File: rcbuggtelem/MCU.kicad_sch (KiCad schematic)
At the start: 12 parts, among them J3 Micro_SD_Card, J4 USB_B_Micro, U1 ESP32-S3-MINI-1

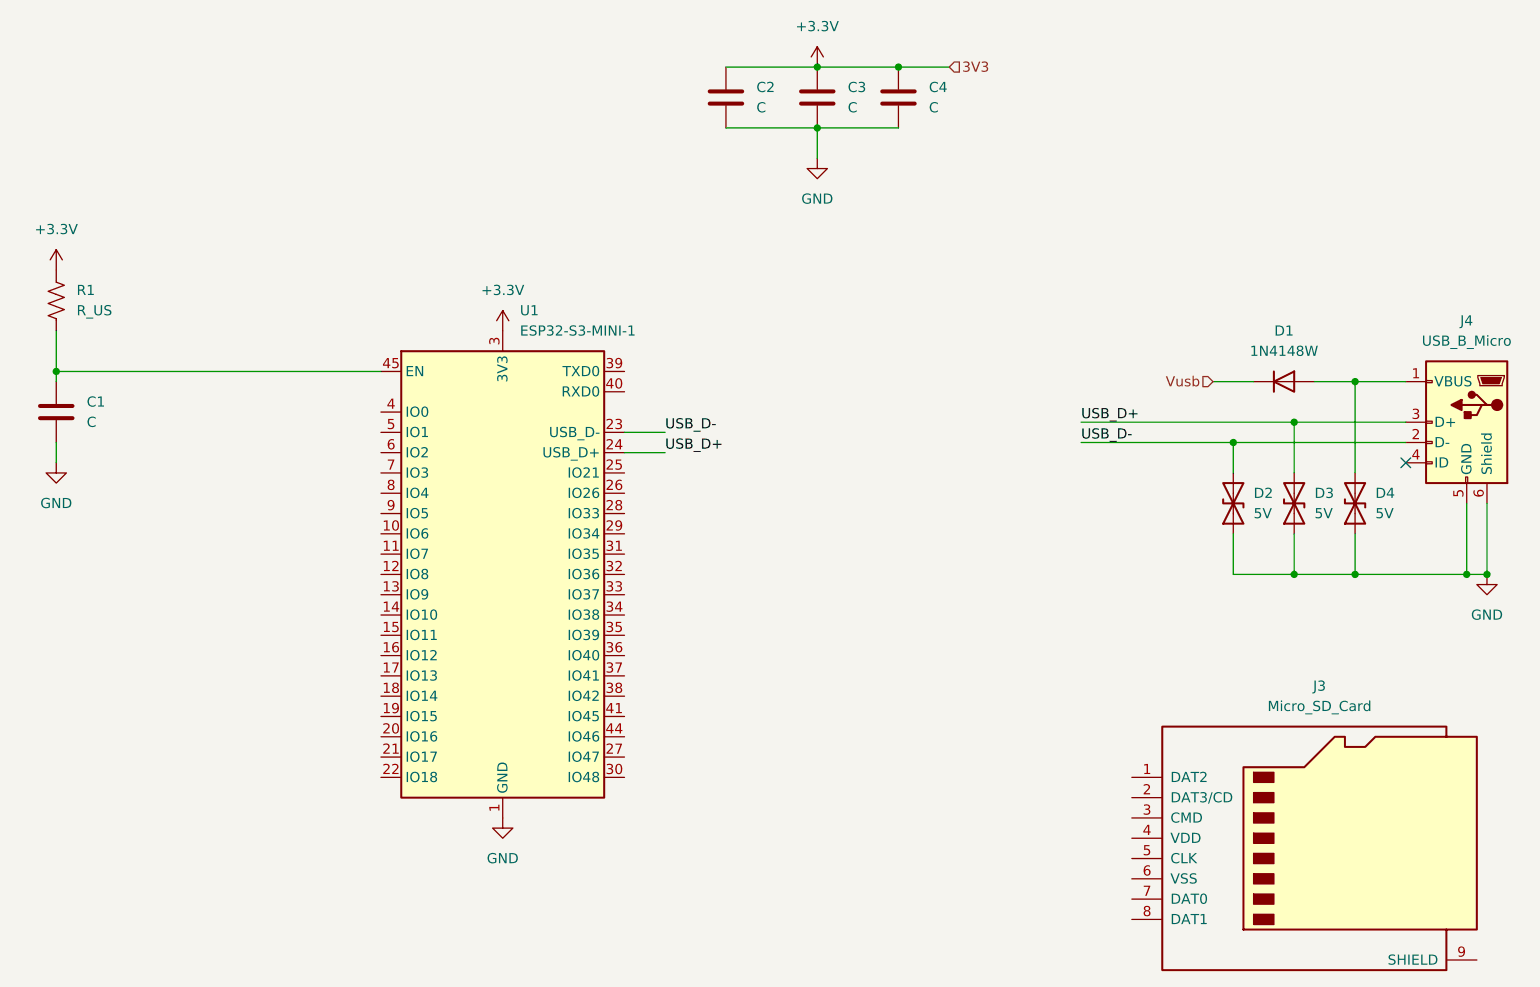
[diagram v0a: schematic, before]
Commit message: Signed-off-by: tom <visentin.tom@gmail.com>
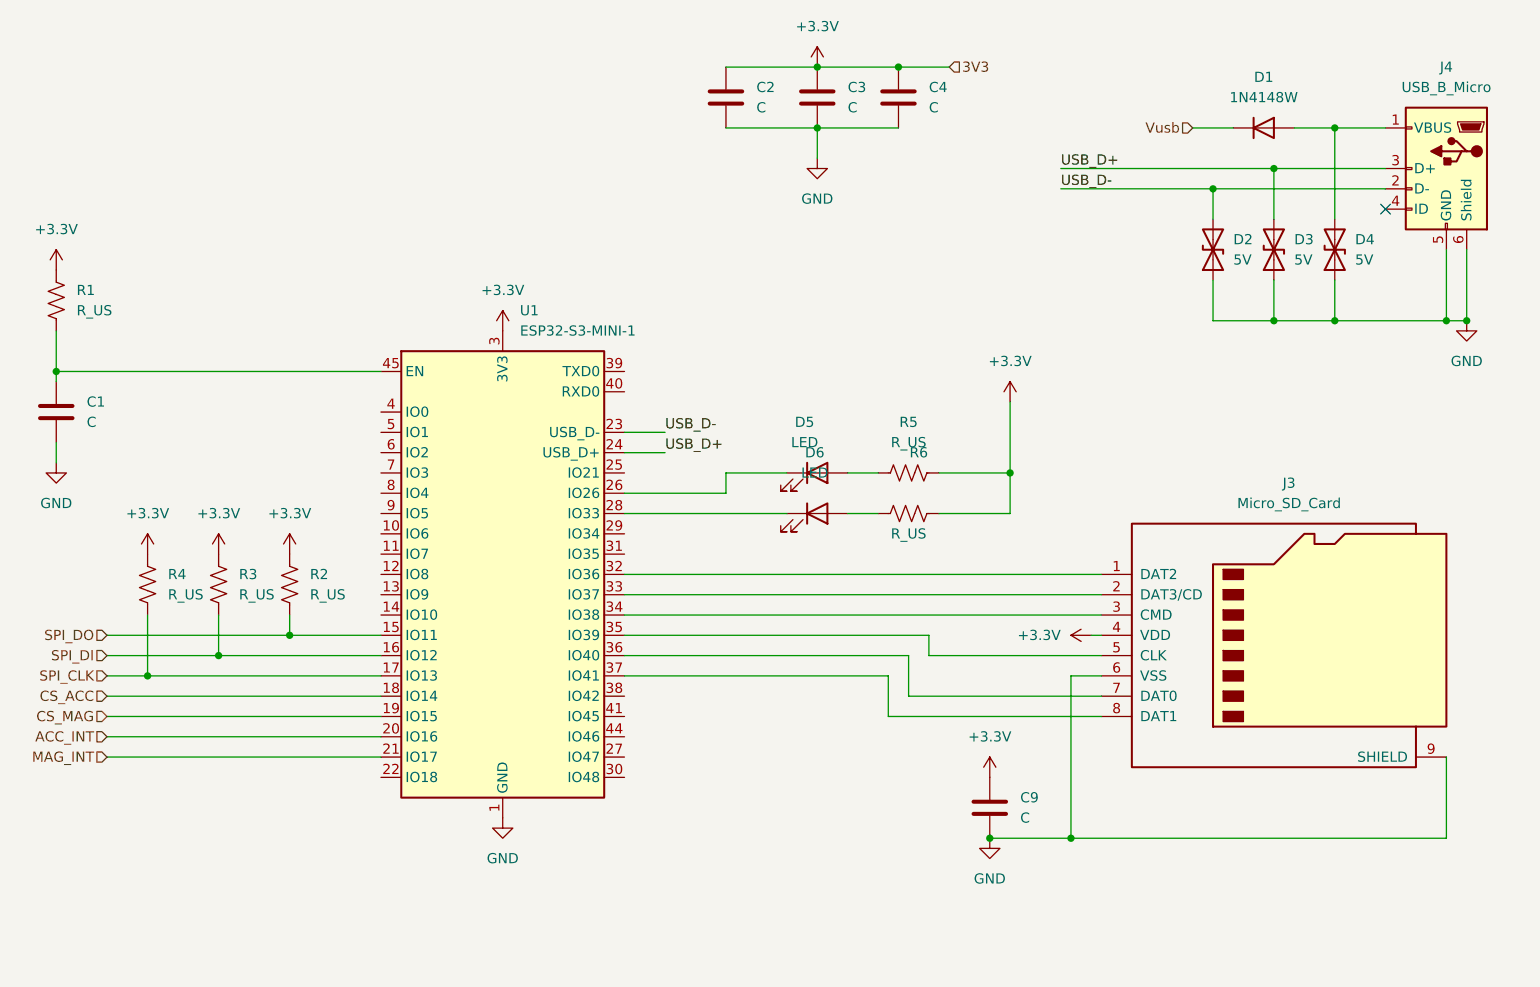
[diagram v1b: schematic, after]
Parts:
- added C9: C, symbol Device:C
- added D5: LED, LED_SMD:LED_0603_1608Metric_Pad1.05x0.95mm_HandSolder, symbol Device:LED
- added D6: LED, symbol Device:LED
- added R2, R3, R4, R5, R6: R_US, symbol Device:R_US
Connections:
- net +3.3V: now also J3.4 (VDD), C9.1, R2.1, R3.1, R4.1, R5.2, R6.2
- net GND: now also J3.6 (VSS), J3.9 (SHIELD), C9.2
- net SPI_DO: now reaches U1.15 (IO11)
- net SPI_DO: now also R2.2
- net SPI_DI: now reaches U1.16 (IO12)
- net SPI_DI: now also R3.2
- net SPI_CLK: now reaches U1.17 (IO13)
- net SPI_CLK: now also R4.2
- net CS_ACC: now reaches U1.18 (IO14)
- net CS_MAG: now reaches U1.19 (IO15)
- net ACC_INT: now reaches U1.20 (IO16)
- net MAG_INT: now reaches U1.21 (IO17)
- net at U1.26 (IO26): now also D5.1 (K)
- net at U1.28 (IO33): now also D6.1 (K)
- net at U1.32 (IO36): now also J3.1 (DAT2)
- net at U1.33 (IO37): now also J3.2 (DAT3/CD)
- net at U1.34 (IO38): now also J3.3 (CMD)
- net at U1.35 (IO39): now also J3.5 (CLK)
- net at U1.36 (IO40): now also J3.7 (DAT0)
- net at U1.37 (IO41): now also J3.8 (DAT1)
- new net: D5.2 (A), R5.1
- new net: D6.2 (A), R6.1
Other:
- moved on the sheet: D1, D2, D3, D4, J3, J4
